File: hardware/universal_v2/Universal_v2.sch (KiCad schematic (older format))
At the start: 14 parts, among them J1 DS18B20, J2 DEV_PORT, J4 Ext, U1 HolyIot-18010, U2 BME680, U3 SHT30-DIS-B

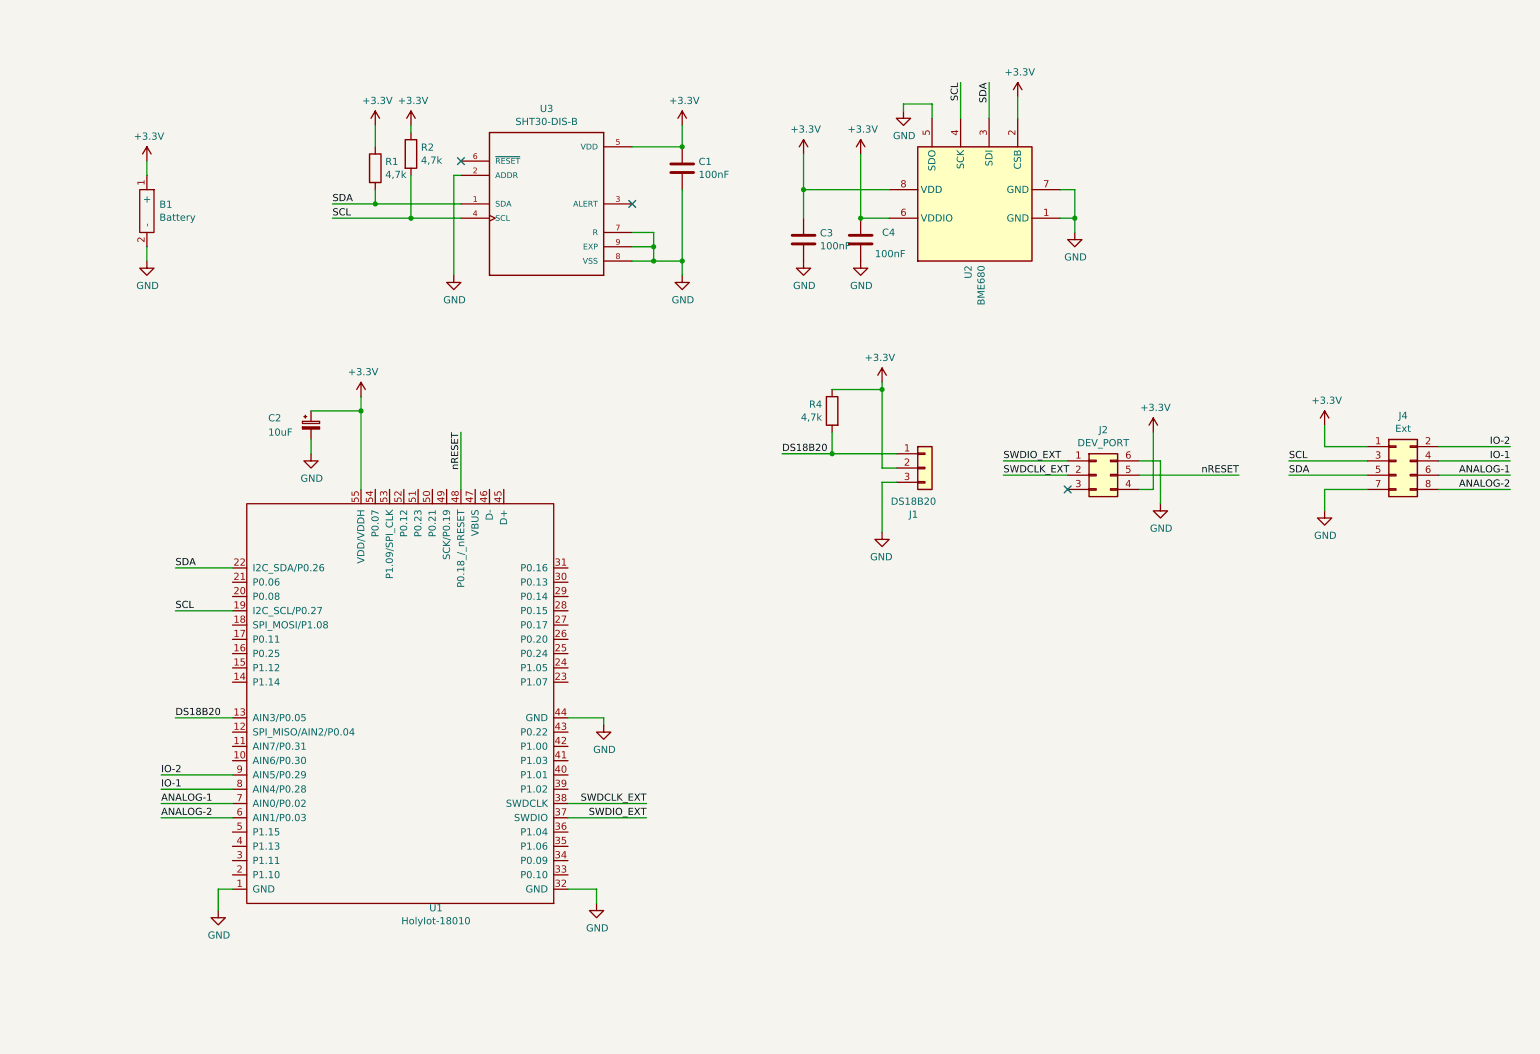
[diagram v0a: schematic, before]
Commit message: Hardware v2, upgrade
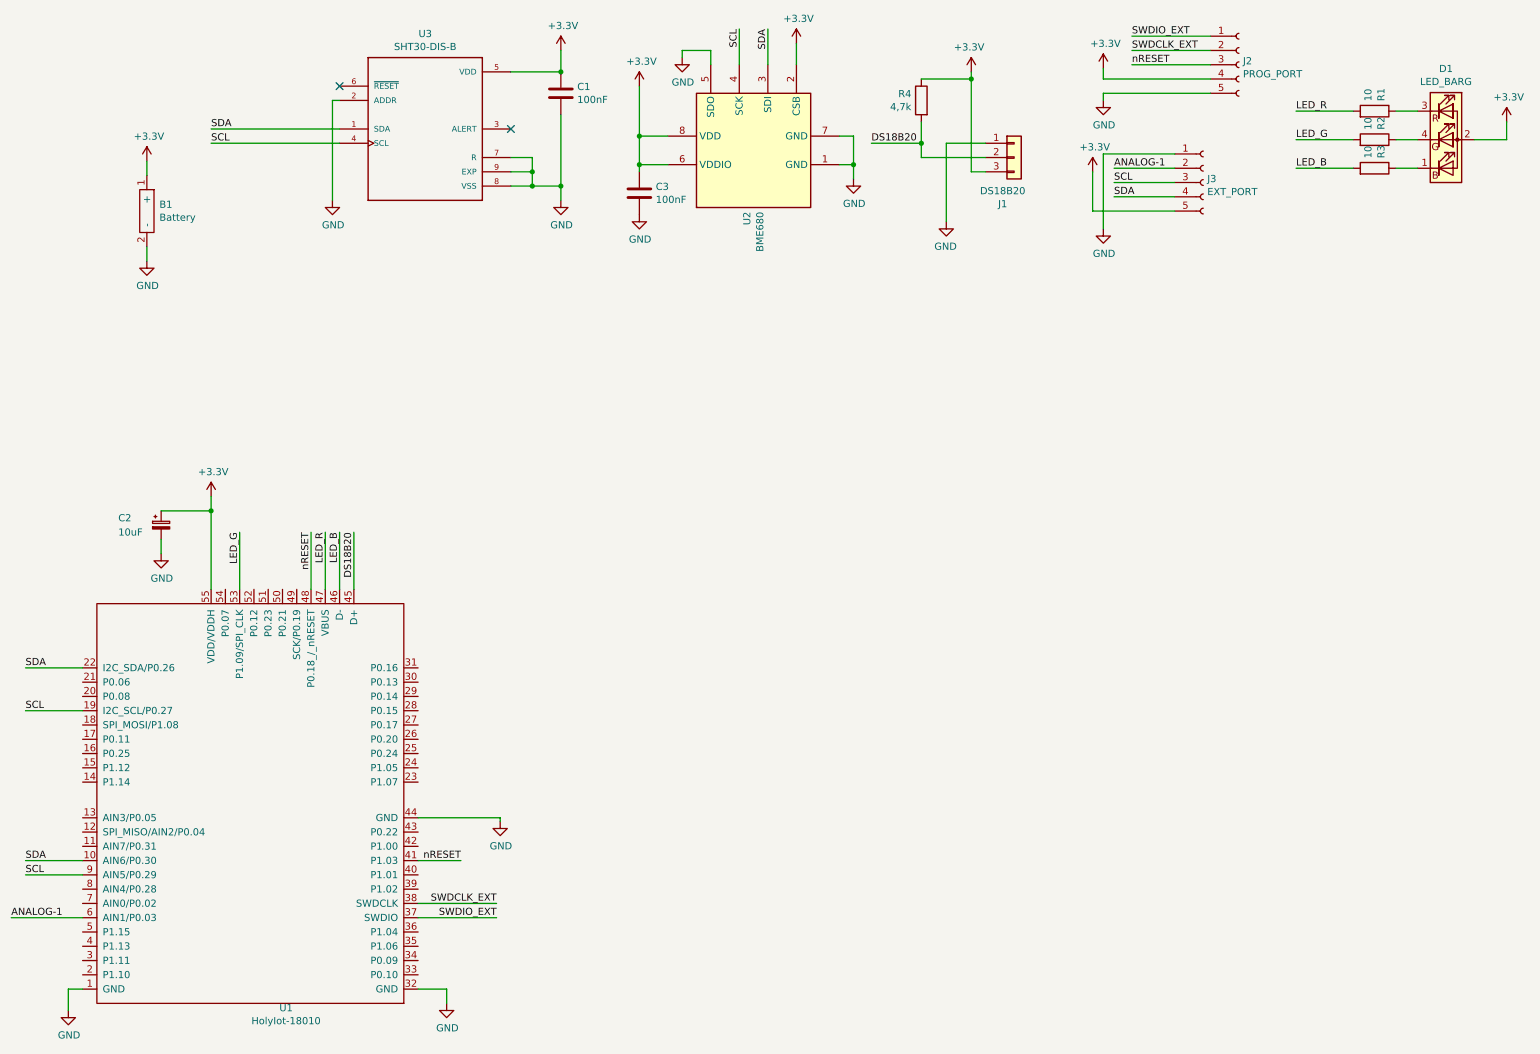
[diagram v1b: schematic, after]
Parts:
- removed C4: 100nF, Capacitor_SMD:C_0402_1005Metric, symbol Device:C
- removed J2: DEV_PORT, Connector_PinHeader_2.54mm:PinHeader_2x03_P2.54mm_Vertical, symbol Connector_Generic:Conn_02x03_Counter_Clockwise
- removed J4: Ext, Connector_PinHeader_1.00mm:PinHeader_2x04_P1.00mm_Vertical_SMD, symbol Connector_Generic:Conn_02x04_Odd_Even
- added D1: LED_BARG, Everlight:Everlight_19-237_R6GHBHC-M07_2T, symbol Device:LED_BARG
- added J2: PROG_PORT, Pads:5xPad, symbol Connector:Conn_01x05_Female
- added J3: EXT_PORT, Pads:5xPad, symbol Connector:Conn_01x05_Female
- added R3: 10, Resistor_SMD:R_0402_1005Metric, symbol Device:R
- R1, R2: value 4,7k -> 10
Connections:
- net ANALOG-2 is gone; now on net ANALOG-1: U1.6 (AIN1/P0.03)
- net IO-2 is gone; now on net SCL: U1.9 (AIN5/P0.29)
- net +3V3: now also J1.3 (Pin_3), D1.2 (A), J2.4 (Pin_4), J3.5 (Pin_5); no longer J1.2 (Pin_2), R1.1, R2.1
- net ANALOG-1: now also J3.2 (Pin_2); no longer U1.7 (AIN0/P0.02)
- net DS18B20: now also J1.2 (Pin_2), U1.45 (D+); no longer J1.1 (Pin_1), U1.13 (AIN3/P0.05)
- net GND: now also J1.1 (Pin_1), J2.5 (Pin_5), J3.1 (Pin_1); no longer J1.3 (Pin_3)
- net SCL: now also J3.3 (Pin_3); no longer R2.2
- net SDA: now also U1.10 (AIN6/P0.30), J3.4 (Pin_4); no longer R1.2
- net SWDCLK_EXT: now also J2.2 (Pin_2)
- net SWDIO_EXT: now also J2.1 (Pin_1)
- net nRESET: now also U1.41 (P1.03), J2.3 (Pin_3)
- net LED_B: now reaches U1.46 (D-)
- net LED_B: now also R3.2
- net LED_R: now reaches U1.47 (VBUS)
- net LED_R: now also R1.2
- net LED_G: now reaches U1.53 (P1.09/SPI_CLK)
- net LED_G: now also R2.2
- net IO-1: no longer names the net of U1.8 (AIN4/P0.28)
- new net: D1.1 (BK), R3.1
- new net: D1.3 (RK), R1.1
- new net: D1.4 (GK), R2.1
- no-connect marks 3 -> 2
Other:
- moved on the sheet: C1, C2, C3, J1, R4, U1, U2, U3
